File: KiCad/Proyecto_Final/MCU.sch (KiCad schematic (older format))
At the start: 112 parts, among them J10 PF, J11 PB, J12 PE, J13 PA, J14 PD, J15 SPI4, J16 OutEn, J17 CFG_SEL, J18 CTRL_MODE, J3 5v, J4 I2C1, J5 ARM SWD, J6 USB_B_Micro, J7 Boot_Select, J8 PG, J9 PC, SW1 Reset, U11 TLV1117-33, U12 USBLC6-2SC6, U13 STM32F723ZCTx, U14 5P49V5929, Y1 25MHz

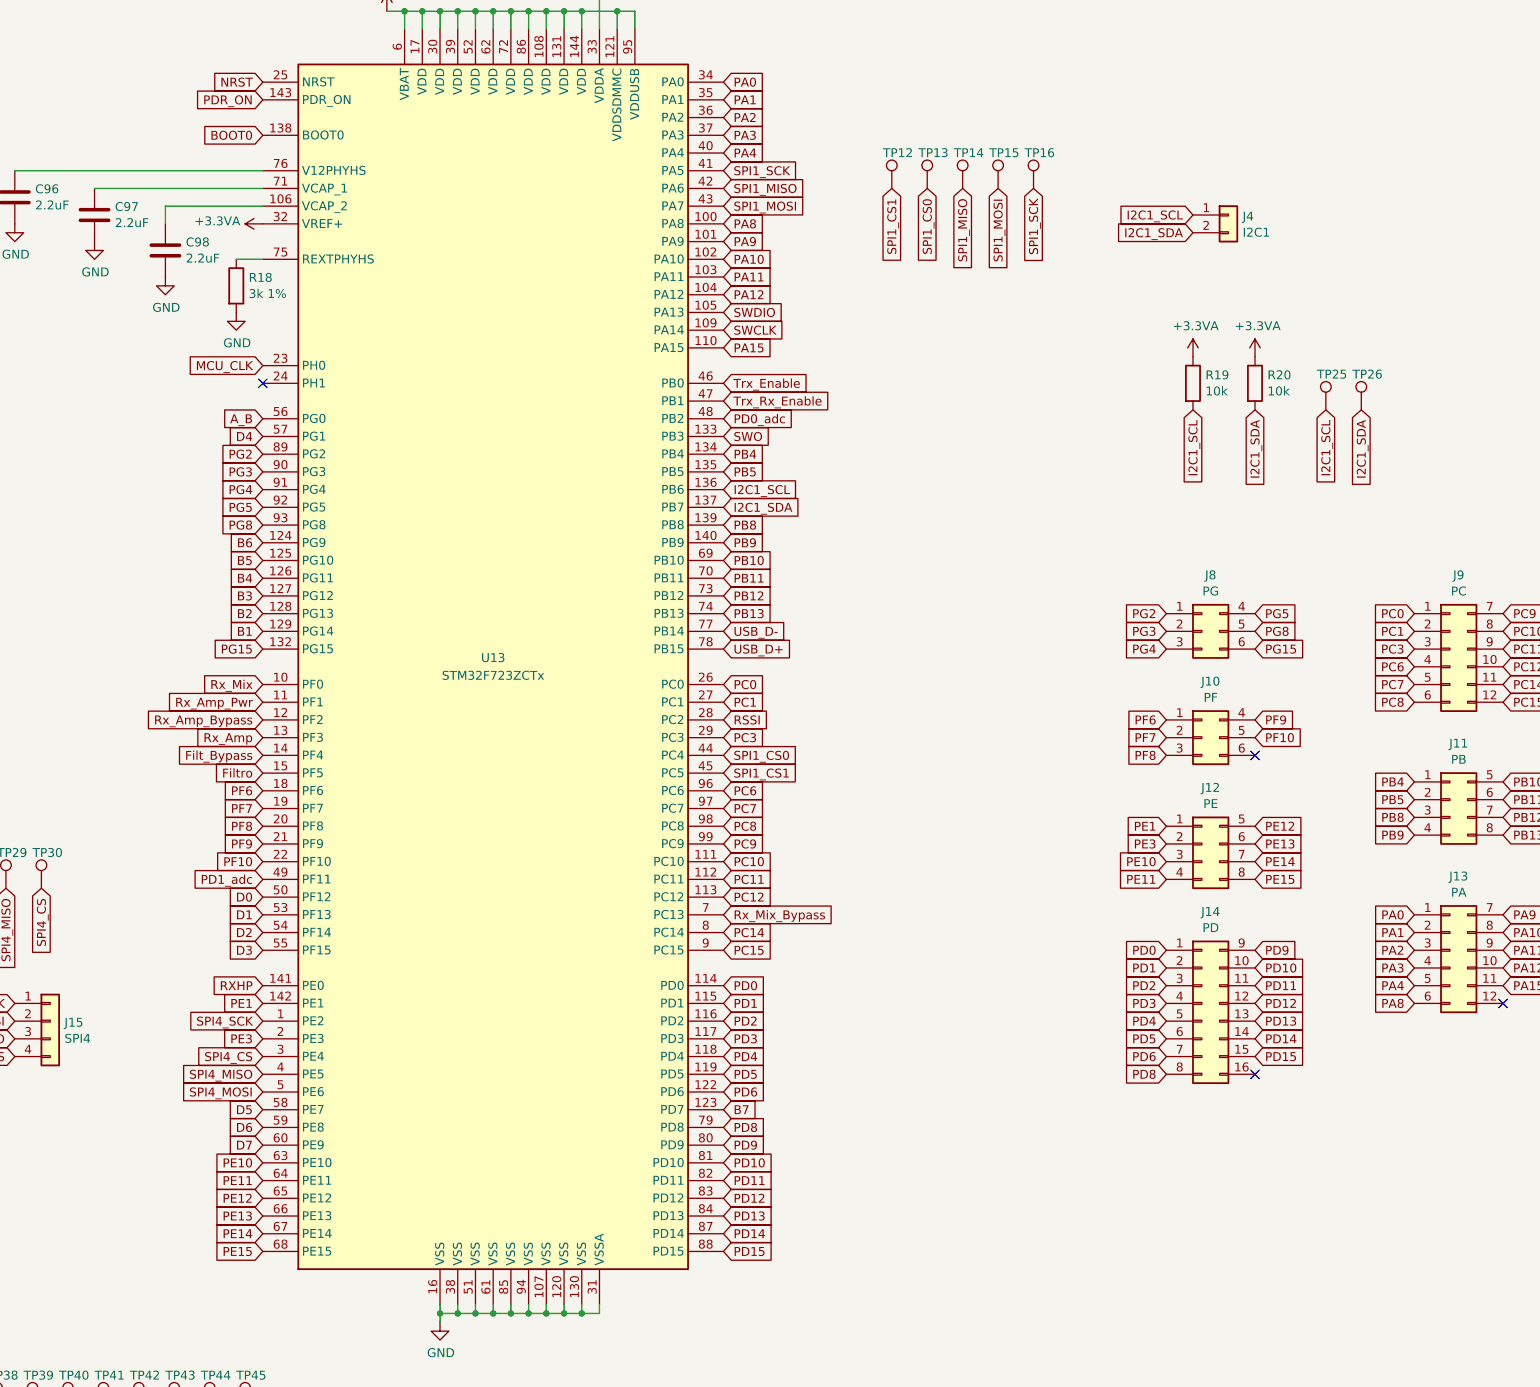
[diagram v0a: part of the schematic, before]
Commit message: Avance PCB.
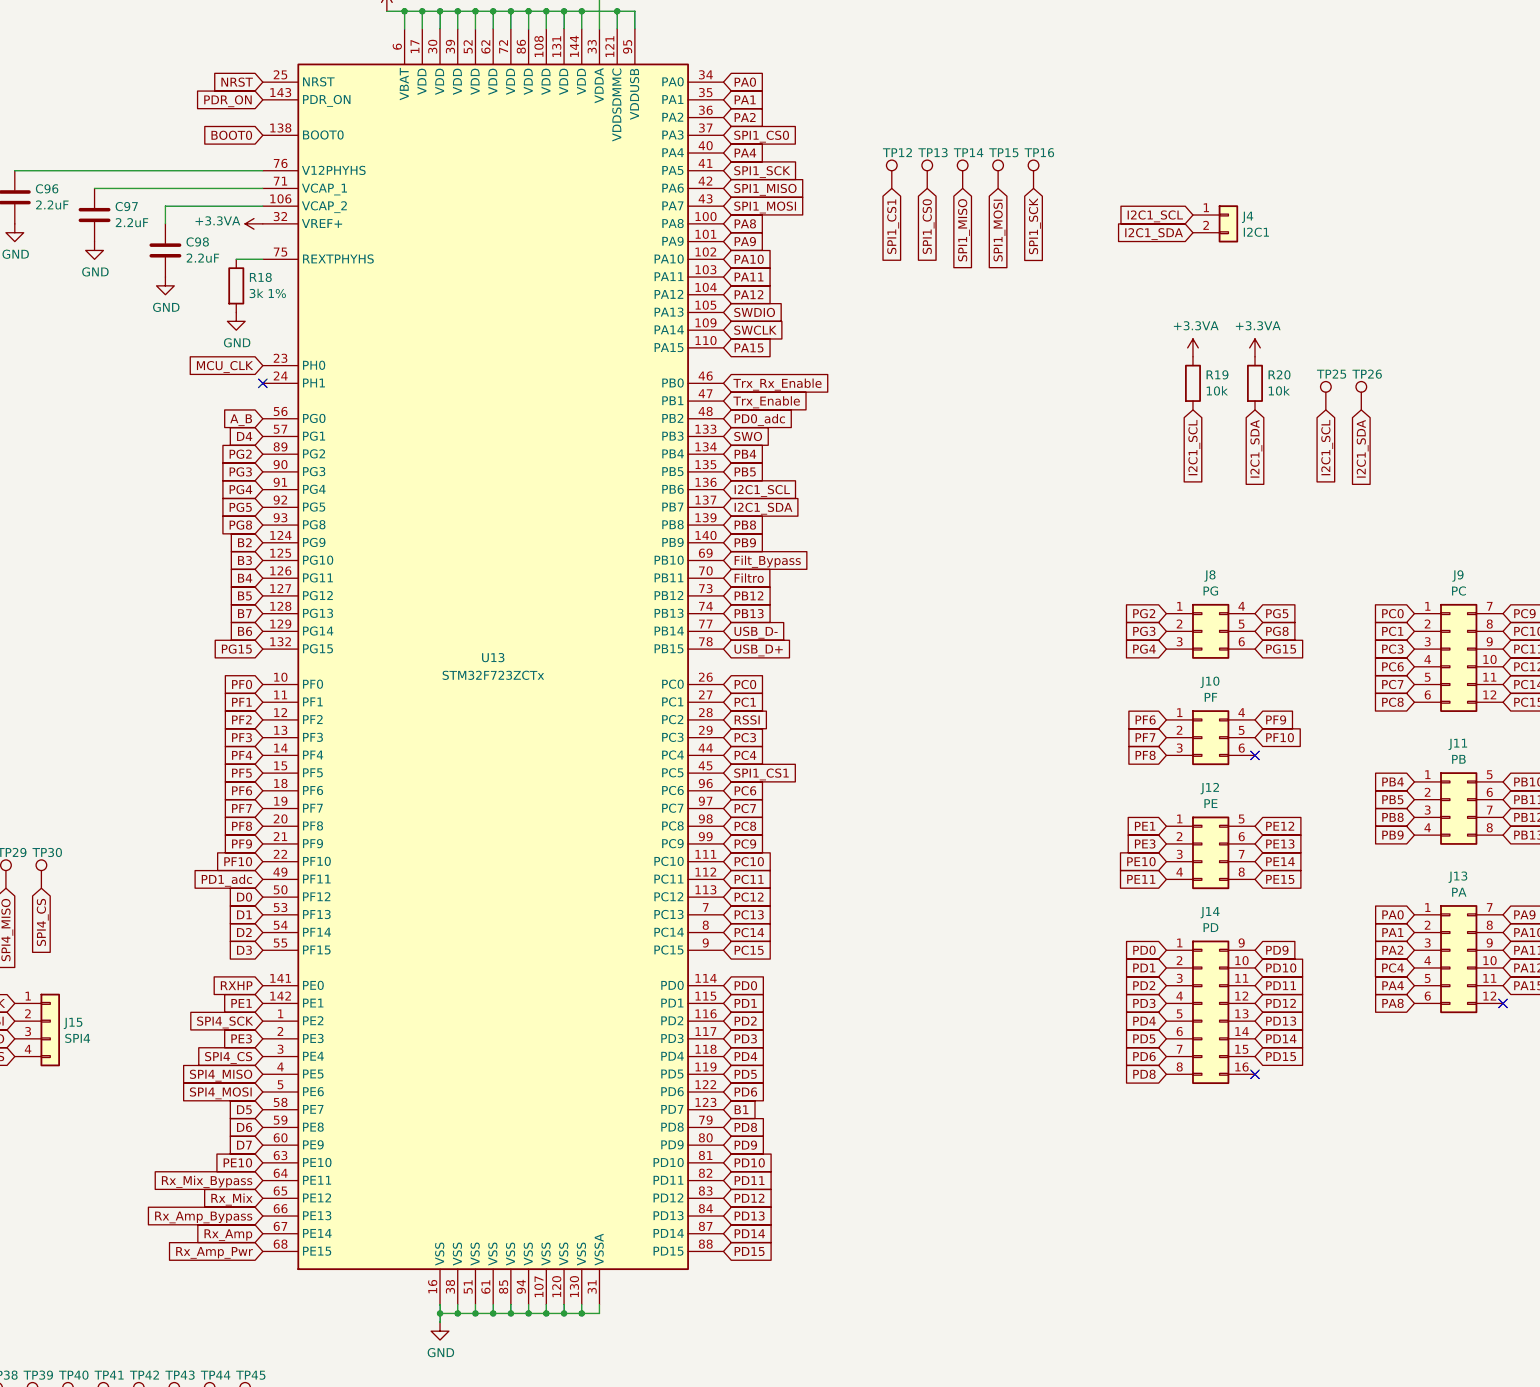
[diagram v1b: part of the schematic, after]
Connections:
- net B1: now also U13.123 (PD7); no longer U13.129 (PG14)
- net B2: now also U13.124 (PG9); no longer U13.128 (PG13)
- net B3: now also U13.125 (PG10); no longer U13.127 (PG12)
- net B5: now also U13.127 (PG12); no longer U13.125 (PG10)
- net B6: now also U13.129 (PG14); no longer U13.124 (PG9)
- net B7: now also U13.128 (PG13); no longer U13.123 (PD7)
- net Filt_Bypass: now also U13.69 (PB10); no longer U13.14 (PF4)
- net Filtro: now also U13.70 (PB11); no longer U13.15 (PF5)
- net PB10: no longer U13.69 (PB10)
- net PB11: no longer U13.70 (PB11)
- net PE11: no longer U13.64 (PE11)
- net PE12: no longer U13.65 (PE12)
- net PE13: no longer U13.66 (PE13)
- net PE14: no longer U13.67 (PE14)
- net PE15: no longer U13.68 (PE15)
- net Rx_Amp: now also U13.67 (PE14); no longer U13.13 (PF3)
- net Rx_Amp_Bypass: now also U13.66 (PE13); no longer U13.12 (PF2)
- net Rx_Amp_Pwr: now also U13.68 (PE15); no longer U13.11 (PF1)
- net Rx_Mix: now also U13.65 (PE12); no longer U13.10 (PF0)
- net Rx_Mix_Bypass: now also U13.64 (PE11); no longer U13.7 (PC13)
- net SPI1_CS0: now also U13.37 (PA3); no longer U13.44 (PC4)
- net Trx_Enable: now also U13.47 (PB1); no longer U13.46 (PB0)
- net Trx_Rx_Enable: now also U13.46 (PB0); no longer U13.47 (PB1)
- net PA3 renamed PC4
- net PC4: now also U13.44 (PC4); no longer U13.37 (PA3)
- new net PC13: U13.7 (PC13)
- new net PF0: U13.10 (PF0)
- new net PF1: U13.11 (PF1)
- new net PF2: U13.12 (PF2)
- new net PF3: U13.13 (PF3)
- new net PF4: U13.14 (PF4)
- new net PF5: U13.15 (PF5)
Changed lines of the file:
@@
 Text GLabel 10450 3350 2    50   Input ~ 0
 SPI1_MOSI
-Text GLabel 10450 6450 2    50   Input ~ 0
+Text GLabel 10450 2950 2    50   Input ~ 0
 SPI1_CS0
 Text GLabel 10450 6550 2    50   Input ~ 0
@@
 Text GLabel 10450 5050 2    50   Input ~ 0
 I2C1_SDA
-Text GLabel 7850 6550 0    50   Input ~ 0
+Text GLabel 10450 5450 2    50   Input ~ 0
 Filtro
-Text GLabel 7850 6450 0    50   Input ~ 0
+Text GLabel 10450 5350 2    50   Input ~ 0
 Filt_Bypass
-Text GLabel 7850 6350 0    50   Input ~ 0
+Text GLabel 7850 9150 0    50   Input ~ 0
 Rx_Amp
-Text GLabel 7850 6250 0    50   Input ~ 0
+Text GLabel 7850 9050 0    50   Input ~ 0
 Rx_Amp_Bypass
-Text GLabel 7850 6150 0    50   Input ~ 0
+Text GLabel 7850 9250 0    50   Input ~ 0
 Rx_Amp_Pwr
-Text GLabel 7850 6050 0    50   Input ~ 0
+Text GLabel 7850 8950 0    50   Input ~ 0
 Rx_Mix
-Text GLabel 10450 7350 2    50   Input ~ 0
+Text GLabel 7850 8850 0    50   Input ~ 0
 Rx_Mix_Bypass
 $Comp
@@
 	5800 3900 5900 3900
 Connection ~ 5900 3900
+Text GLabel 10450 4450 2    50   Input ~ 0
+Trx_Enable
 Text GLabel 10450 4350 2    50   Input ~ 0
-Trx_Enable
-Text GLabel 10450 4450 2    50   Input ~ 0
 Trx_Rx_Enable
 Text GLabel 10450 6250 2    50   Input ~ 0
@@
 Text GLabel 7850 7750 0    50   Input ~ 0
 RXHP
-Text GLabel 7850 5750 0    50   Input ~ 0
+Text GLabel 10450 8450 2    50   Input ~ 0
 B1
-Text GLabel 7850 5650 0    50   Input ~ 0
+Text GLabel 7850 5250 0    50   Input ~ 0
 B2
-Text GLabel 7850 5550 0    50   Input ~ 0
+Text GLabel 7850 5350 0    50   Input ~ 0
 B3
 Text GLabel 7850 5450 0    50   Input ~ 0
 B4
-Text GLabel 7850 5350 0    50   Input ~ 0
+Text GLabel 7850 5550 0    50   Input ~ 0
 B5
-Text GLabel 7850 5250 0    50   Input ~ 0
+Text GLabel 7850 5750 0    50   Input ~ 0
 B6
-Text GLabel 10450 8450 2    50   Input ~ 0
+Text GLabel 7850 5650 0    50   Input ~ 0
 B7
 $Comp
@@
 Text GLabel 7850 8750 0    50   Input ~ 0
 PE10
-Text GLabel 7850 8850 0    50   Input ~ 0
-PE11
-Text GLabel 7850 8950 0    50   Input ~ 0
-PE12
-Text GLabel 7850 9050 0    50   Input ~ 0
-PE13
-Text GLabel 7850 9150 0    50   Input ~ 0
-PE14
-Text GLabel 7850 9250 0    50   Input ~ 0
-PE15
+Text GLabel 10450 7350 2    50   Input ~ 0
+PC13
+Text GLabel 7850 6050 0    50   Input ~ 0
+PF0
+Text GLabel 7850 6250 0    50   Input ~ 0
+PF2
+Text GLabel 7850 6350 0    50   Input ~ 0
+PF3
+Text GLabel 7850 6150 0    50   Input ~ 0
+PF1
 Text GLabel 12950 6850 0    50   Input ~ 0
 PE1
@@
 Text GLabel 10450 5250 2    50   Input ~ 0
 PB9
-Text GLabel 10450 5350 2    50   Input ~ 0
-PB10
-Text GLabel 10450 5450 2    50   Input ~ 0
-PB11
+Text GLabel 7850 6450 0    50   Input ~ 0
+PF4
+Text GLabel 7850 6550 0    50   Input ~ 0
+PF5
 Text GLabel 10450 5550 2    50   Input ~ 0
 PB12
@@
 Text GLabel 10450 3050 2    50   Input ~ 0
 PA4
-Text GLabel 10450 2950 2    50   Input ~ 0
-PA3
+Text GLabel 10450 6450 2    50   Input ~ 0
+PC4
 Text GLabel 10450 2850 2    50   Input ~ 0
 PA2
@@
 Text GLabel 14350 7750 0    50   Input ~ 0
 PA4
-Text GLabel 14350 7650 0    50   Input ~ 0
-PA3
 Text GLabel 14350 7550 0    50   Input ~ 0
 PA2
@@
 	1    0    0    -1
 $EndComp
+Text GLabel 14350 7650 0    50   Input ~ 0
+PC4
 $EndSCHEMATC
